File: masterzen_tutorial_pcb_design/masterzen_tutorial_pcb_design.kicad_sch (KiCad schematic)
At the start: 18 parts, among them J1 AVR-ISP-6, U1 ATmega32U4-A, Y1 Crystal_GND24_Small

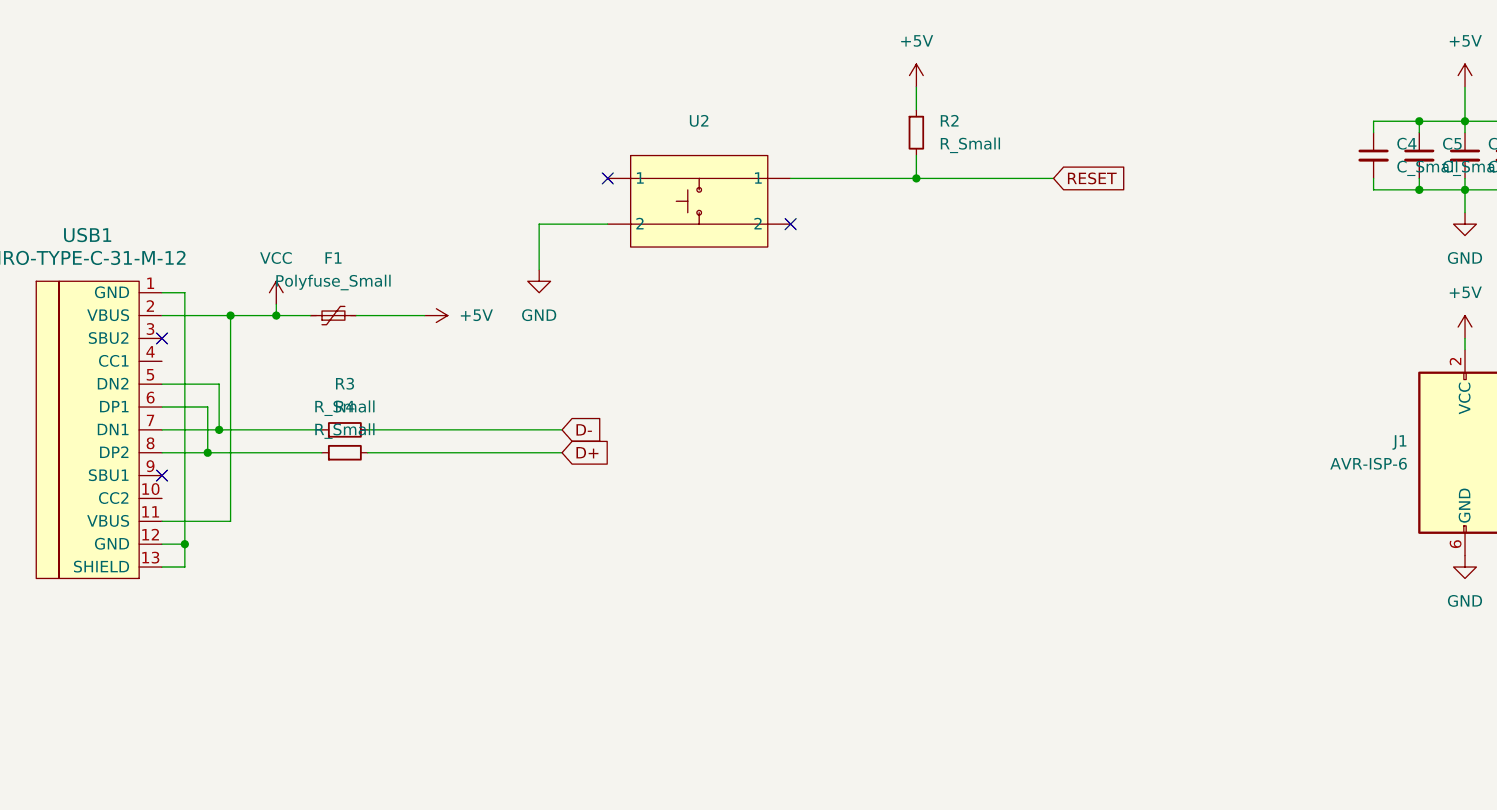
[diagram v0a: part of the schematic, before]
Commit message: finished part 1
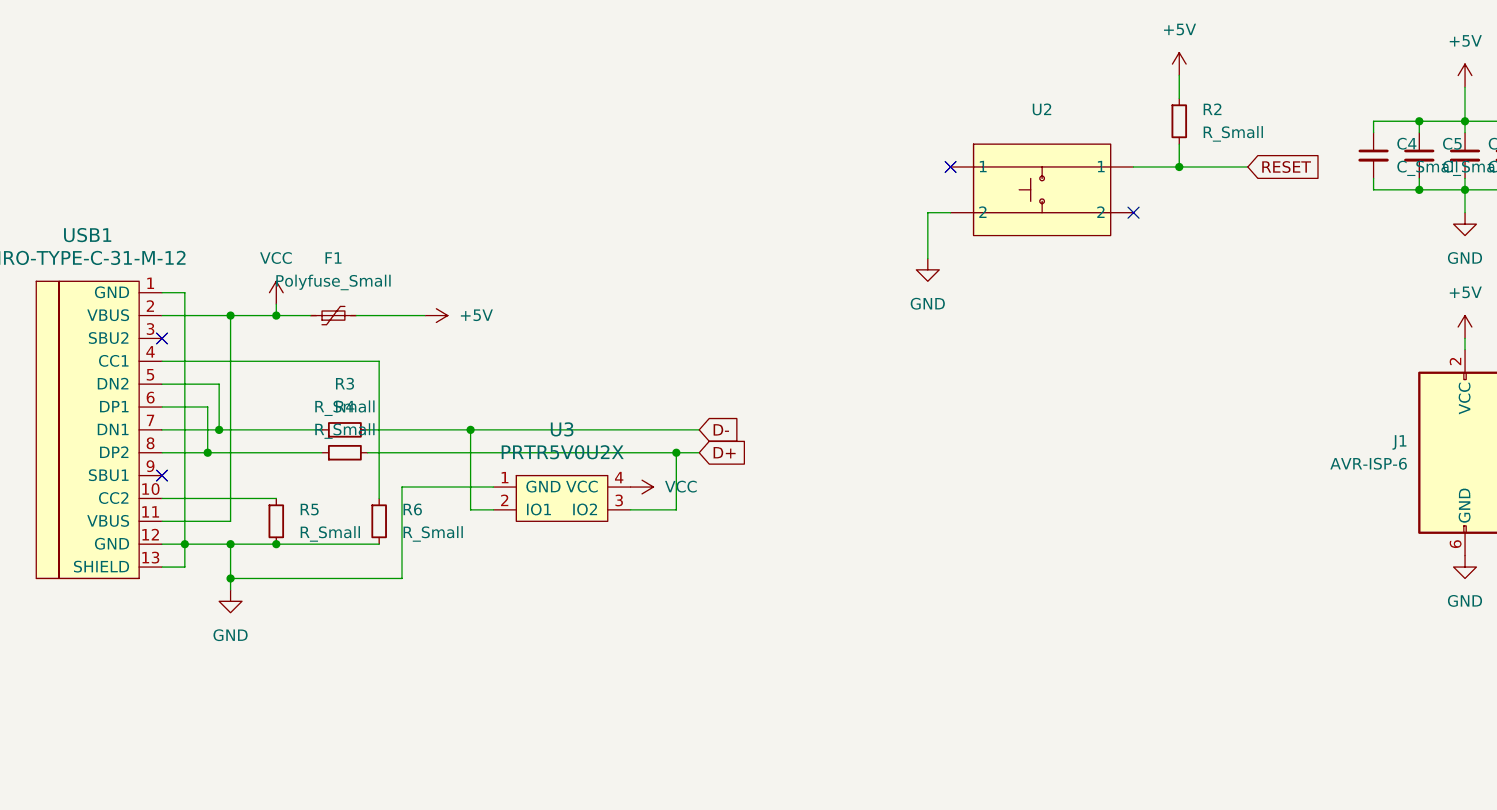
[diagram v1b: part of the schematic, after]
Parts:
- added R5, R6: R_Small, symbol Device:R_Small
- added U3: PRTR5V0U2X, symbol random-keyboard-parts:PRTR5V0U2X
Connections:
- net D+: now also U3.3 (IO2)
- net D-: now also U3.2 (IO1)
- net GND: now also USB1.1 (GND), USB1.12 (GND), USB1.13 (SHIELD), R5.2, R6.2, U3.1 (GND)
- net VCC: now also U3.4 (VCC)
- net at USB1.10 (CC2): now also R5.1
- net at USB1.4 (CC1): now also R6.1
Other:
- moved on the sheet: R2, U2

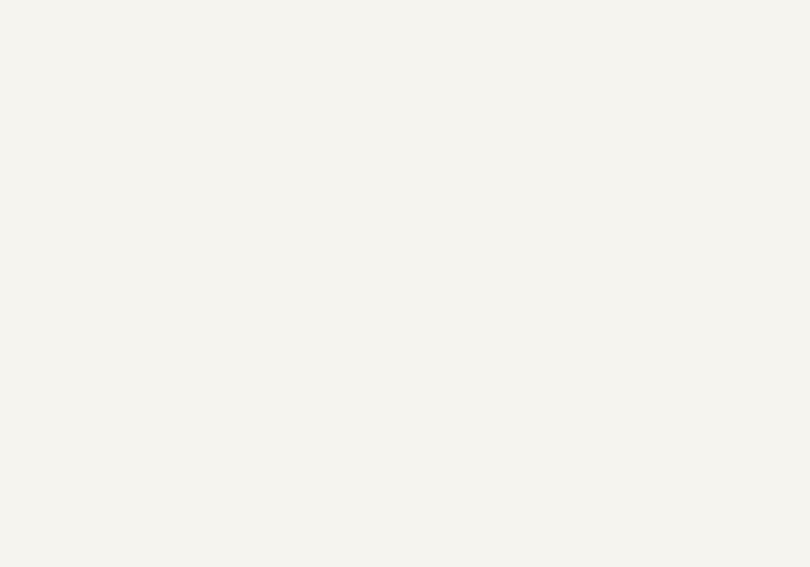
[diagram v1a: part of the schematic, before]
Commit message: initial matrix
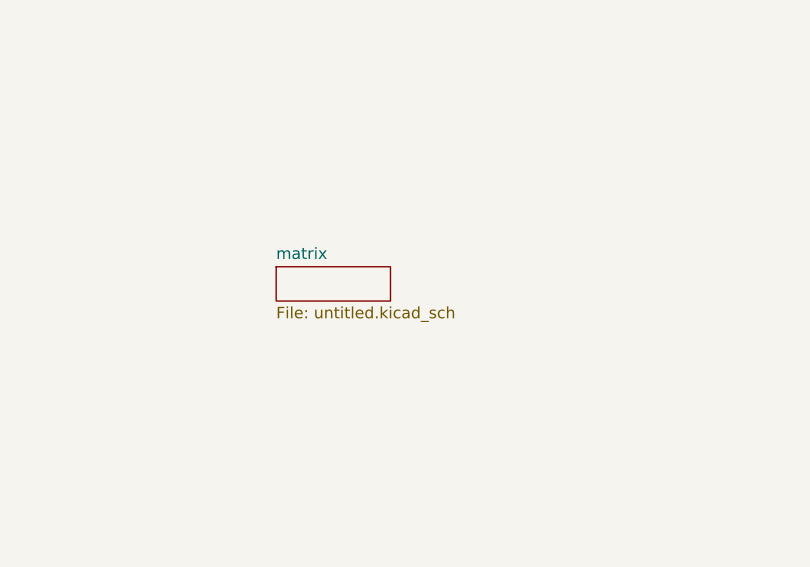
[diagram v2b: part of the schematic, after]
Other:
- added sheet matrix (untitled.kicad_sch)
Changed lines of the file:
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@@
+		)
+	)
+	(sheet
+		(at 96.52 104.14)
+		(size 12.7 3.81)
+		(fields_autoplaced yes)
+		(stroke
+			(width 0.1524)
+			(type solid)
+		)
+		(fill
+			(color 0 0 0 0.0000)
+		)
+		(property "Sheetname" "matrix"
+			(at 96.52 103.4284 0)
+			(effects
+				(font
+					(size 1.27 1.27)
+				)
+				(justify left bottom)
+			)
+		)
+		(property "Sheetfile" "untitled.kicad_sch"
+			(at 96.52 108.5346 0)
+			(effects
+				(font
+					(size 1.27 1.27)
+				)
+				(justify left top)
+			)
+		)
+		(instances
+			(project "masterzen_tutorial_pcb_design"
+				(path "/43ab7f41-8dc3-471f-b30f-d5100c2539fd"
+					(page "2")
+				)
+			)
 		)
 	)
